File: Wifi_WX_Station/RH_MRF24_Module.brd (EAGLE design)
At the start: 23.2 x 33.6 mm, 7 parts, among them M1 MRF24WB0MA

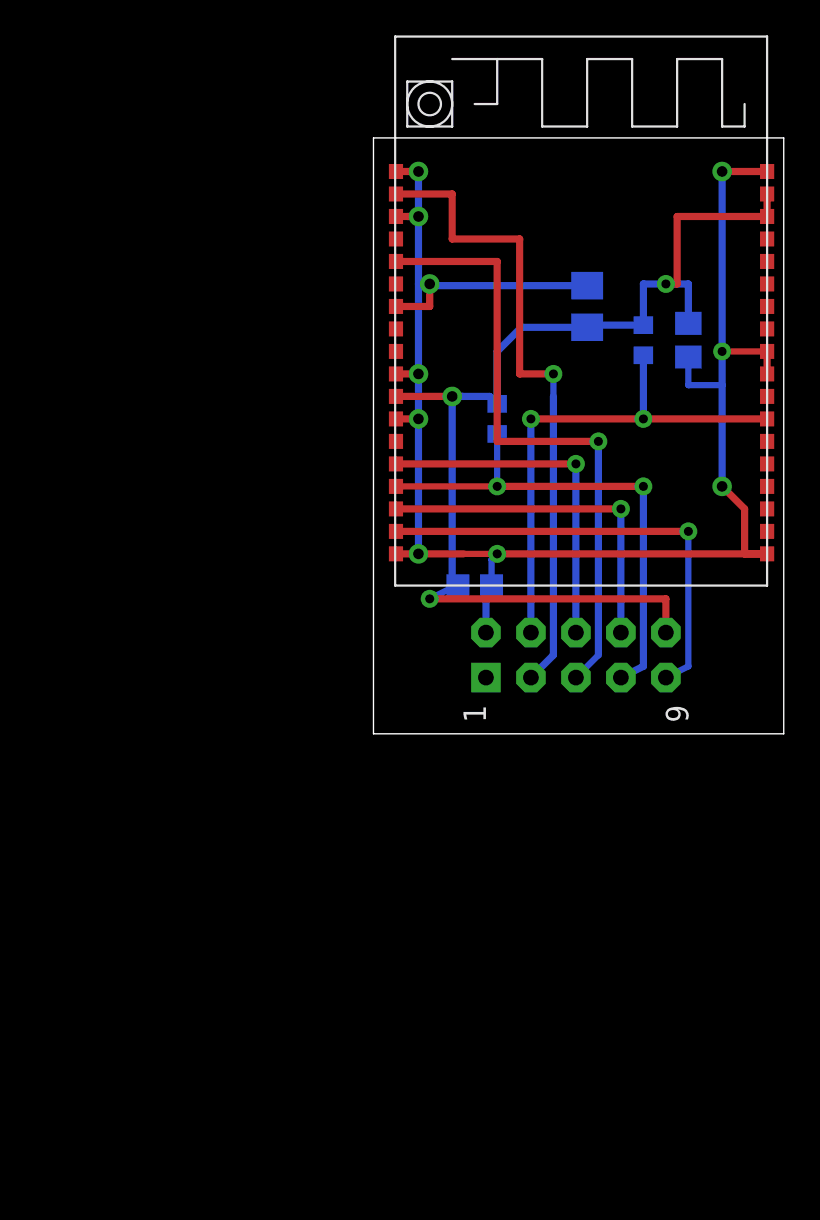
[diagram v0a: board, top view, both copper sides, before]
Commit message: updated BOM with all prices- As Checked in to BATCH PCB
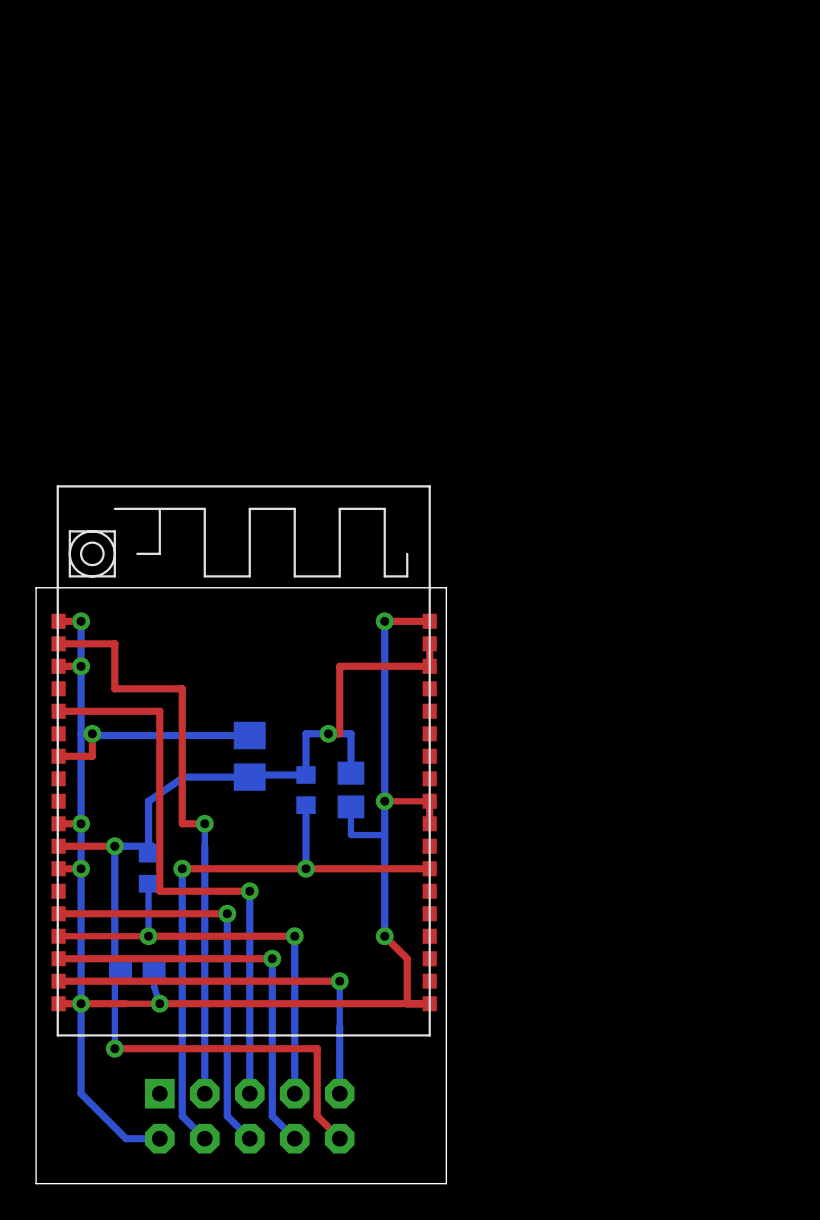
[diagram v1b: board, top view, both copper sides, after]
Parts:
- moved R1 32.1 mm to (8.26, 19.1)
- moved JP1 31.9 mm to (14.0, 5.08), flipped to the bottom, turned to 270 degrees
- moved M1 31.8 mm to (24.1, 40.6)
- moved C2 31.8 mm to (19.7, 23.5)
- moved C3 31.8 mm to (14.0, 25.4)
- moved R2 31.8 mm to (17.1, 23.5)
- moved C1 28.8 mm to (7.62, 13.3)
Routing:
- net GND: track 99.1 -> 106.8 mm
- net RESET_: track 29.0 -> 33.3 mm
- net INT_: track 28.5 -> 25.2 mm
- net SDI: track 25.5 -> 22.2 mm
- net SDO: track 19.7 -> 22.8 mm
- net SCK: track 19.7 -> 22.8 mm
- net CS_: track 35.5 -> 32.4 mm
- net HIBER: track 36.7 -> 33.7 mm
- net +3V3: track 64.1 -> 65.5 mm
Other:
- board text removed: "0.5080 mm / 20.000 mil"
- board text removed: "0.6000 mm / 23.622 mil"
- board text removed: "0.8890 mm / 35.000 mil"
- board text removed: "1 different diameters with default symbols! (10 drills)"
- board text removed: "Date: 1/27/2013 12:40:03 PM"
- board text removed: "Drill legend"
